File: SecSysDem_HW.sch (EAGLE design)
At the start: 56 parts, among them IC1 L7805 5V, Q1 2N3904, T1 MOSFET_NCHANNEL_ENHANCEMENT2N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, T2 MOSFET_NCHANNEL_ENHANCEMENT2N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, T3 MOSFET_NCHANNEL_ENHANCEMENT2N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, U1 XPLAINED_MINI_PINOUT, U2 PCF8574_IO_EXPANDER, U4 FT24C512A, U5 MCP4901-E/SN, X1 C-GRID-06-70553, X5 C-GRID-02-70543, X7 C-GRID-02-70543, X8 C-GRID-02-70543

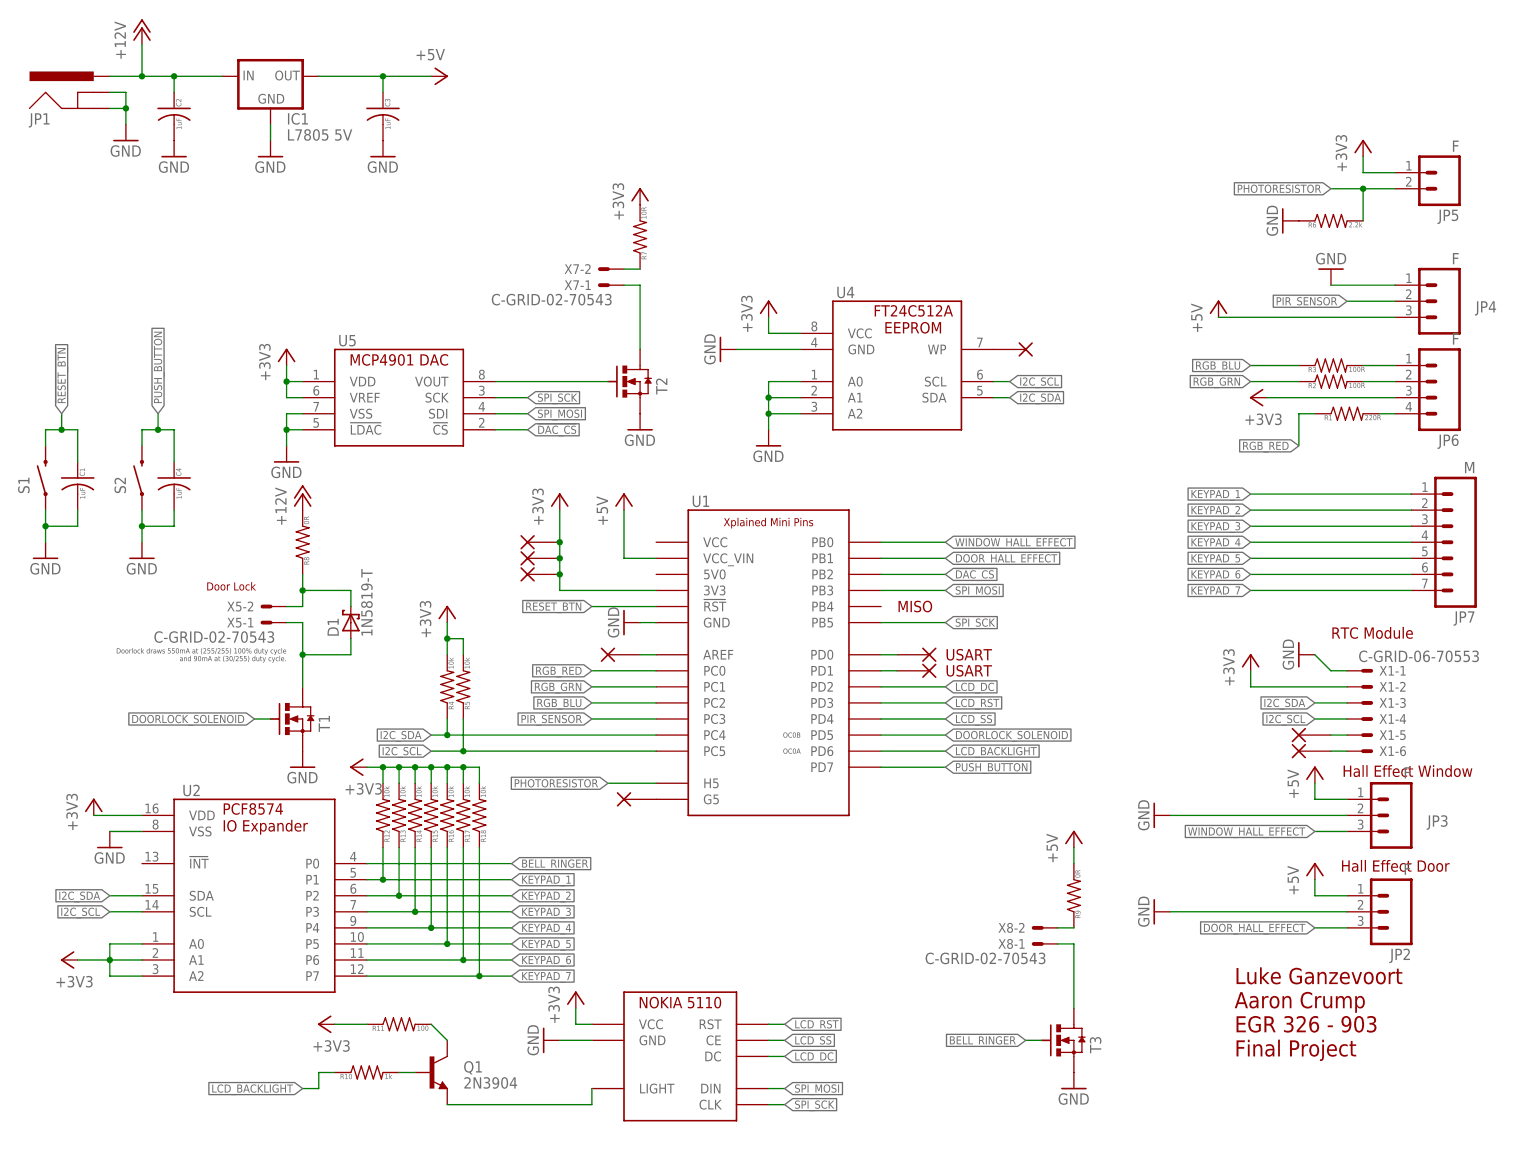
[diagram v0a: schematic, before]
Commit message: Made board mods to schematic
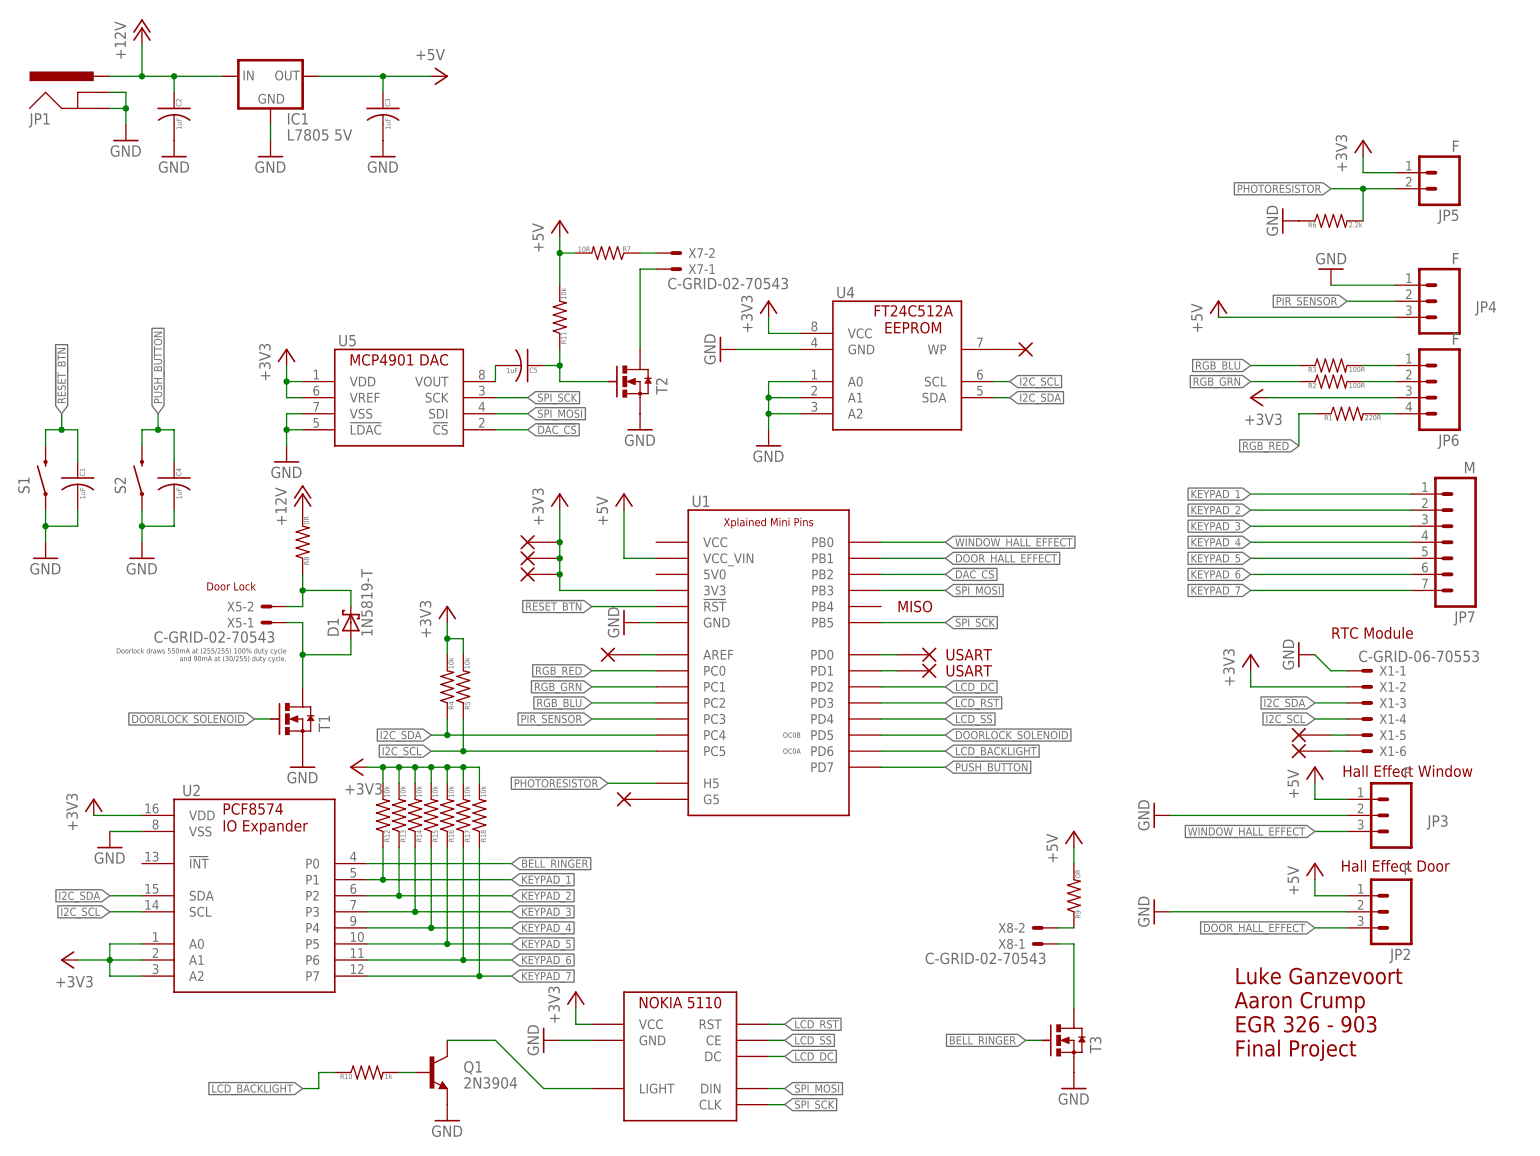
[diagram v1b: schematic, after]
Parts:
- added C5: 1uF, Luke:CAPACITOR0805
- R11: value 100 -> 10k
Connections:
- net +3V3: no longer R11.1, R7.2
- net +5V: now also R11.2, R7.2
- net GND: now also Q1.E
- net N$18: now also U$3.LIGHT; no longer R11.2
- net N$19: now also C5.NEG, U5.VOUT; no longer Q1.E, U$3.LIGHT
- net N$3: now also C5.POS, R11.1; no longer U5.VOUT
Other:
- moved on the sheet: R11, R7, X7-1, X7-2
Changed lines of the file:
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@@
 <part name="R7" library="Luke" deviceset="RESISTOR" device="0805" value="10R"/>
 <part name="X7" library="con-molex" deviceset="C-GRID-02" device="-70543"/>
-<part name="+3V8" library="supply1" deviceset="+3V3" device=""/>
 <part name="U4" library="Luke" deviceset="FT24C512A" device=""/>
 <part name="+3V9" library="supply1" deviceset="+3V3" device=""/>
@@
 <part name="+3V11" library="supply1" deviceset="+3V3" device=""/>
 <part name="Q1" library="SparkFun-DiscreteSemi" deviceset="TRANSISTOR_NPN" device="BC547" value="2N3904"/>
-<part name="+3V12" library="supply1" deviceset="+3V3" device=""/>
 <part name="R10" library="Luke" deviceset="RESISTOR" device="0805" value="1k"/>
-<part name="R11" library="Luke" deviceset="RESISTOR" device="0805" value="100"/>
 <part name="+3V13" library="supply1" deviceset="+3V3" device=""/>
 <part name="D1" library="diode" deviceset="1N581*" device="" technology="9-T"/>
@@
 <part name="+3V14" library="supply1" deviceset="+3V3" device=""/>
 <part name="P+8" library="supply1" deviceset="+5V" device=""/>
+<part name="GND3" library="supply1" deviceset="GND" device=""/>
+<part name="P+9" library="supply1" deviceset="+5V" device=""/>
+<part name="R11" library="Luke" deviceset="RESISTOR" device="0805" value="10k"/>
+<part name="C5" library="Luke" deviceset="CAPACITOR" device="0805" value="1uF"/>
 </parts>
 <sheets>
@@
 <instance part="T2" gate="G$1" x="104.14" y="124.46"/>
 <instance part="GND18" gate="1" x="104.14" y="116.84"/>
-<instance part="R7" gate="G$1" x="104.14" y="147.32" rot="R90"/>
-<instance part="X7" gate="-2" x="99.06" y="142.24" rot="R180"/>
-<instance part="X7" gate="-1" x="99.06" y="139.7" rot="R180"/>
-<instance part="+3V8" gate="G$1" x="104.14" y="154.94"/>
+<instance part="R7" gate="G$1" x="99.06" y="144.78" rot="R180"/>
+<instance part="X7" gate="-2" x="109.22" y="144.78" rot="MR180"/>
+<instance part="X7" gate="-1" x="109.22" y="142.24" rot="MR180"/>
 <instance part="U4" gate="G$1" x="134.62" y="116.84"/>
 <instance part="+3V9" gate="G$1" x="124.46" y="137.16"/>
@@
 <instance part="+3V11" gate="G$1" x="218.44" y="162.56"/>
 <instance part="Q1" gate="G$1" x="71.12" y="15.24"/>
-<instance part="+3V12" gate="G$1" x="53.34" y="22.86" rot="R90"/>
 <instance part="R10" gate="G$1" x="60.96" y="15.24"/>
-<instance part="R11" gate="G$1" x="66.04" y="22.86"/>
 <instance part="+3V13" gate="G$1" x="12.7" y="33.02" rot="R90"/>
 <instance part="D1" gate="G$1" x="58.42" y="86.36" rot="R90"/>
@@
 <instance part="+3V14" gate="G$1" x="58.42" y="63.5" rot="R90"/>
 <instance part="P+8" gate="1" x="172.72" y="53.34"/>
+<instance part="GND3" gate="1" x="73.66" y="7.62"/>
+<instance part="P+9" gate="1" x="91.44" y="149.86"/>
+<instance part="R11" gate="G$1" x="91.44" y="134.62" rot="R90"/>
+<instance part="C5" gate="G$1" x="86.36" y="127" rot="R270"/>
 </instances>
 <busses>
@@
 <pinref part="GND21" gate="1" pin="GND"/>
 </segment>
+<segment>
+<pinref part="Q1" gate="G$1" pin="E"/>
+<pinref part="GND3" gate="1" pin="GND"/>
+</segment>
 </net>
 <net name="I2C_SDA" class="0">
@@
 <wire x1="172.72" y1="50.8" x2="172.72" y2="48.26" width="0.1524" layer="91"/>
 <pinref part="P+8" gate="1" pin="+5V"/>
+</segment>
+<segment>
+<pinref part="R7" gate="G$1" pin="2"/>
+<pinref part="P+9" gate="1" pin="+5V"/>
+<wire x1="93.98" y1="144.78" x2="91.44" y2="144.78" width="0.1524" layer="91"/>
+<wire x1="91.44" y1="144.78" x2="91.44" y2="147.32" width="0.1524" layer="91"/>
+<pinref part="R11" gate="G$1" pin="2"/>
+<wire x1="91.44" y1="139.7" x2="91.44" y2="144.78" width="0.1524" layer="91"/>
+<junction x="91.44" y="144.78"/>
 </segment>
 </net>
@@
 </segment>
 <segment>
-<pinref part="+3V8" gate="G$1" pin="+3V3"/>
-<pinref part="R7" gate="G$1" pin="2"/>
-</segment>
-<segment>
 <wire x1="223.52" y1="157.48" x2="218.44" y2="157.48" width="0.1524" layer="91"/>
 <wire x1="218.44" y1="157.48" x2="218.44" y2="160.02" width="0.1524" layer="91"/>
 <pinref part="+3V11" gate="G$1" pin="+3V3"/>
 <pinref part="JP5" gate="G$1" pin="1"/>
-</segment>
-<segment>
-<pinref part="R11" gate="G$1" pin="1"/>
-<pinref part="+3V12" gate="G$1" pin="+3V3"/>
-<wire x1="60.96" y1="22.86" x2="55.88" y2="22.86" width="0.1524" layer="91"/>
 </segment>
 <segment>
@@
 <net name="N$3" class="0">
 <segment>
-<wire x1="81.28" y1="124.46" x2="99.06" y2="124.46" width="0.1524" layer="91"/>
 <pinref part="T2" gate="G$1" pin="G"/>
-<pinref part="U5" gate="G$1" pin="VOUT"/>
+<pinref part="R11" gate="G$1" pin="1"/>
+<wire x1="91.44" y1="127" x2="91.44" y2="124.46" width="0.1524" layer="91"/>
+<wire x1="91.44" y1="124.46" x2="99.06" y2="124.46" width="0.1524" layer="91"/>
+<wire x1="91.44" y1="129.54" x2="91.44" y2="127" width="0.1524" layer="91"/>
+<pinref part="C5" gate="G$1" pin="POS"/>
+<wire x1="91.44" y1="127" x2="88.9" y2="127" width="0.1524" layer="91"/>
+<junction x="91.44" y="127"/>
 </segment>
 </net>
@@
 <segment>
 <pinref part="X7" gate="-2" pin="S"/>
-<wire x1="101.6" y1="142.24" x2="104.14" y2="142.24" width="0.1524" layer="91"/>
+<wire x1="106.68" y1="144.78" x2="104.14" y2="144.78" width="0.1524" layer="91"/>
 <pinref part="R7" gate="G$1" pin="1"/>
 </segment>
@@
 <pinref part="X7" gate="-1" pin="S"/>
 <pinref part="T2" gate="G$1" pin="D"/>
-<wire x1="101.6" y1="139.7" x2="104.14" y2="139.7" width="0.1524" layer="91"/>
-<wire x1="104.14" y1="139.7" x2="104.14" y2="129.54" width="0.1524" layer="91"/>
+<wire x1="106.68" y1="142.24" x2="104.14" y2="142.24" width="0.1524" layer="91"/>
+<wire x1="104.14" y1="142.24" x2="104.14" y2="129.54" width="0.1524" layer="91"/>
 </segment>
 </net>
@@
 <pinref part="Q1" gate="G$1" pin="B"/>
 <wire x1="66.04" y1="15.24" x2="68.58" y2="15.24" width="0.1524" layer="91"/>
-</segment>
-</net>
-<net name="N$18" class="0">
-<segment>
-<pinref part="Q1" gate="G$1" pin="C"/>
-<pinref part="R11" gate="G$1" pin="2"/>
-<wire x1="73.66" y1="20.32" x2="71.12" y2="22.86" width="0.1524" layer="91"/>
-</segment>
-</net>
-<net name="N$19" class="0">
-<segment>
-<pinref part="U$3" gate="G$1" pin="LIGHT"/>
-<pinref part="Q1" gate="G$1" pin="E"/>
-<wire x1="96.52" y1="12.7" x2="96.52" y2="10.16" width="0.1524" layer="91"/>
-<wire x1="96.52" y1="10.16" x2="73.66" y2="10.16" width="0.1524" layer="91"/>
 </segment>
 </net>
@@
 </segment>
 </net>
+<net name="N$18" class="0">
+<segment>
+<pinref part="U$3" gate="G$1" pin="LIGHT"/>
+<wire x1="96.52" y1="12.7" x2="88.9" y2="12.7" width="0.1524" layer="91"/>
+<wire x1="88.9" y1="12.7" x2="81.28" y2="20.32" width="0.1524" layer="91"/>
+<pinref part="Q1" gate="G$1" pin="C"/>
+<wire x1="81.28" y1="20.32" x2="73.66" y2="20.32" width="0.1524" layer="91"/>
+</segment>
+</net>
+<net name="N$19" class="0">
+<segment>
+<pinref part="U5" gate="G$1" pin="VOUT"/>
+<pinref part="C5" gate="G$1" pin="NEG"/>
+<wire x1="81.28" y1="127" x2="81.28" y2="124.46" width="0.1524" layer="91"/>
+</segment>
+</net>
